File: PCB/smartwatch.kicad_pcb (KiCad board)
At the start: 2 copper layers, 34.2 x 34.2 mm, 6 parts, among them J1 Conn_01x04_Pin, U1 STM32L432KBUx, U2 LSM6DS3, U3 W25Q128JVPIQ, U4 TP4056

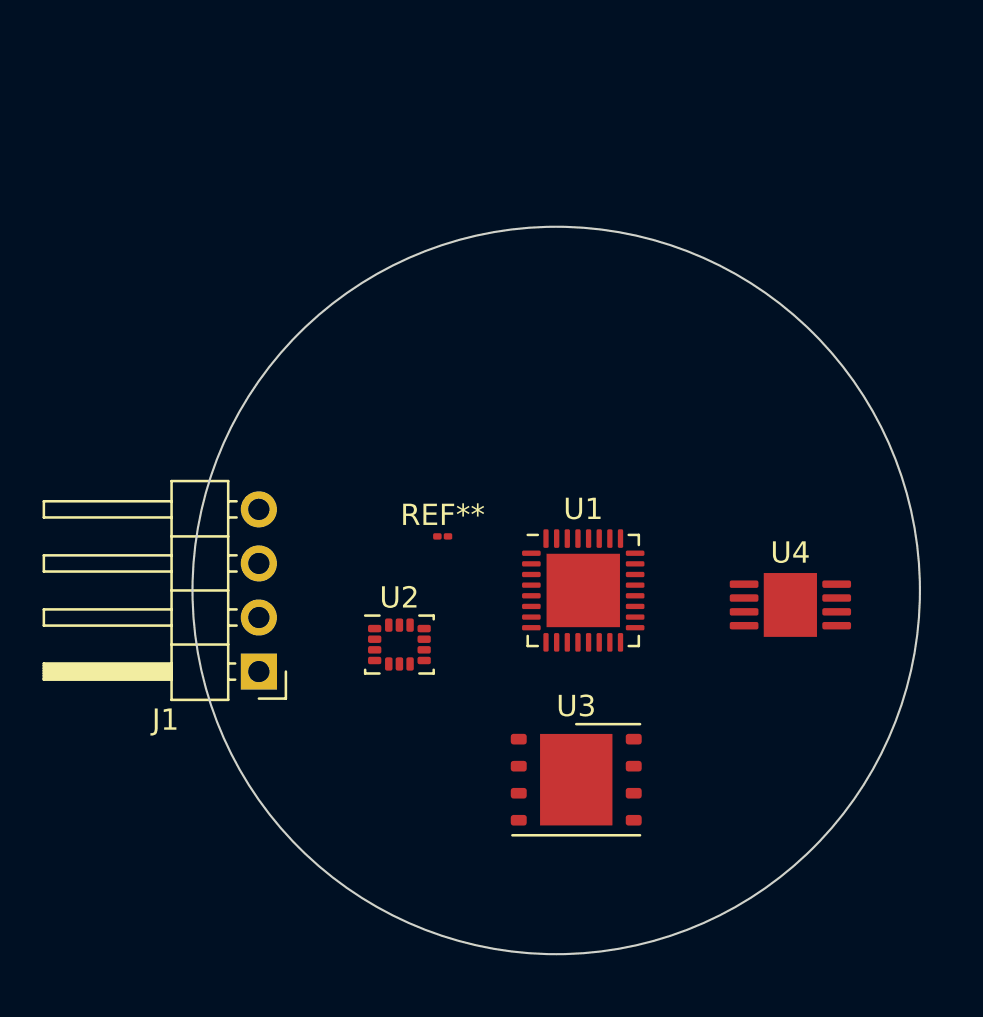
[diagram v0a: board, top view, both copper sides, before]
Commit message: new staffz
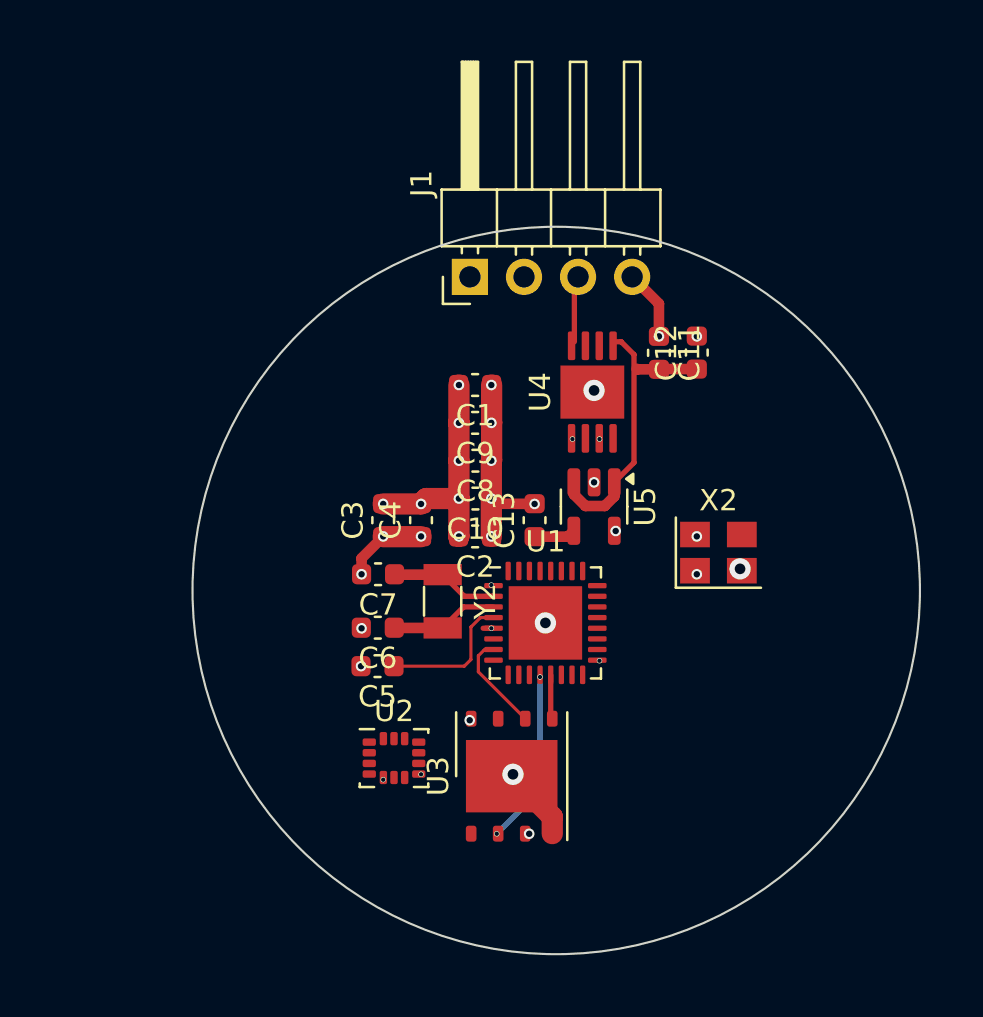
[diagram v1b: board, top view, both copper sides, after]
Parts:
- removed REF**: C_01005_0402Metric, Capacitor_SMD:C_01005_0402Metric
- added C1: 4.7uf, Capacitor_SMD:C_0603_1608Metric, F.Cu at (153.7, 84.3)
- added C10: 100nf, Capacitor_SMD:C_0603_1608Metric, F.Cu at (153.7, 89.7)
- added C11: 4.7uf, Capacitor_SMD:C_0603_1608Metric, F.Cu at (162.3, 82.8)
- added C12: 4.7uf, Capacitor_SMD:C_0603_1608Metric, F.Cu at (164.1, 82.8)
- added C13: 4.7uf, Capacitor_SMD:C_0603_1608Metric, F.Cu at (156.5, 90.7)
- added C2: 100nf, Capacitor_SMD:C_0603_1608Metric, F.Cu at (153.7, 91.4)
- added C3: 100nf, Capacitor_SMD:C_0603_1608Metric, F.Cu at (149.4, 90.7)
- added C4: 100nf, Capacitor_SMD:C_0603_1608Metric, F.Cu at (151.1, 90.7)
- added C5: 100nf, Capacitor_SMD:C_0603_1608Metric, F.Cu at (149.1, 97.5)
- added C6: 9pf, Capacitor_SMD:C_0603_1608Metric, F.Cu at (149.1, 95.7)
- added C7: 9pf, Capacitor_SMD:C_0603_1608Metric, F.Cu at (149.1, 93.2)
- added C8: 100nf, Capacitor_SMD:C_0603_1608Metric, F.Cu at (153.7, 87.9)
- added C9: 100nf, Capacitor_SMD:C_0603_1608Metric, F.Cu at (153.7, 86.1)
- added U5: LT1761-3.3, Package_TO_SOT_SMD:TSOT-23-5, F.Cu at (159.3, 90.0)
- added X2: 20Mhz, Crystal:Crystal_SMD_3225-4Pin_3.2x2.5mm, F.Cu at (165.1, 92.2)
- added Y2: LSE 32khz, Crystal:Crystal_SMD_3215-2Pin_3.2x1.5mm, F.Cu at (152.1, 94.5)
- J1: value Conn_01x04_Pin -> Serial wire/Charging
- moved J1 21.0 mm to (153.4, 79.2), turned to 90 degrees
- moved U4 13.7 mm to (159.2, 84.7), turned to 90 degrees
- moved U2 5.34 mm to (149.9, 101.9)
- moved U3 3.04 mm to (155.4, 102.7), turned to 90 degrees
- moved U1 2.34 mm to (157.0, 95.5)
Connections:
- J1 pad 3: unconnected-(J1-Pin_3-Pad3) -> VIN
- J1 pad 4: unconnected-(J1-Pin_4-Pad4) -> GND
- U1 pad 1: unconnected-(U1-VDD-Pad1) -> VDD
- U1 pad 12: unconnected-(U1-PA6-Pad12) -> SPI1_MISO
- U1 pad 13: unconnected-(U1-PA7-Pad13) -> SPI1_MOSI
- U1 pad 16: Net-(U1-VSS-Pad16) -> GND
- U1 pad 17: unconnected-(U1-VDD-Pad17) -> VDD
- U1 pad 2: unconnected-(U1-PC14-Pad2) -> OSC32_IN
- U1 pad 3: unconnected-(U1-PC15-Pad3) -> OSC32_OUT
- U1 pad 32: Net-(U1-VSS-Pad16) -> GND
- U1 pad 33: Net-(U1-VSS-Pad16) -> GND
- U1 pad 4: unconnected-(U1-NRST-Pad4) -> Net-(U1-NRST)
- U1 pad 5: unconnected-(U1-VDDA-Pad5) -> VDD
- U1 pad 6: unconnected-(U1-PA0-Pad6) -> CLKIN
- U1 pad 7: unconnected-(U1-PA1-Pad7) -> SPI1_SCK
- U2 pad 1: unconnected-(U2-SDO/SA0-Pad1) -> SPI1_MISO
- U2 pad 12: unconnected-(U2-CS-Pad12) -> GYRO_CS
- U2 pad 13: unconnected-(U2-SCL-Pad13) -> SPI1_SCK
- U2 pad 14: unconnected-(U2-SDA-Pad14) -> SPI1_MISO
- U2 pad 2: unconnected-(U2-SDX-Pad2) -> GND
- U2 pad 3: unconnected-(U2-SCX-Pad3) -> GND
- U2 pad 4: unconnected-(U2-INT1-Pad4) -> GYRO_INT1
- U2 pad 5: unconnected-(U2-VDDIO-Pad5) -> VDD
- U2 pad 6: Net-(U2-GND-Pad6) -> GND
- U2 pad 7: Net-(U2-GND-Pad6) -> GND
- U2 pad 8: unconnected-(U2-VDD-Pad8) -> VDD
- U2 pad 9: unconnected-(U2-INT2-Pad9) -> GYRO_INT2
- U3 pad 1: unconnected-(U3-/CS-Pad1) -> FLASH_CS
- U3 pad 2: unconnected-(U3-DO_(IO1)-Pad2) -> SPI1_MISO
- U3 pad 3: unconnected-(U3-/WP_(IO2)-Pad3) -> VDD
- U3 pad 4: (no net) -> GND
- U3 pad 5: unconnected-(U3-DI_(IO0)-Pad5) -> SPI1_MOSI
- U3 pad 6: unconnected-(U3-CLK-Pad6) -> SPI1_SCK
- U3 pad 7: unconnected-(U3-/HOLD_or_/RESET_(IO3)-Pad7) -> HR_FLASH
- U3 pad 8: unconnected-(U3-VCC-Pad8) -> VDD
- U3 pad 9: unconnected-(U3-Pad9) -> GND
- U4 pad 1: unconnected-(U4-TEMP-Pad1) -> GND
- U4 pad 2: unconnected-(U4-PROG-Pad2) -> Net-(U4-PROG)
- U4 pad 3: unconnected-(U4-GND-Pad3) -> GND
- U4 pad 4: unconnected-(U4-VCC-Pad4) -> VIN
- U4 pad 5: unconnected-(U4-BAT-Pad5) -> BAT
- U4 pad 7: unconnected-(U4-~{CHRG}-Pad7) -> CHARGE
- U4 pad 8: unconnected-(U4-CE-Pad8) -> VIN
- U4 pad 9: unconnected-(U4-PP-Pad9) -> GND
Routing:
- net GND: track 0.00 -> 89.1 mm, vias 0 -> 20
- net VDD: track 0.00 -> 70.5 mm, vias 0 -> 17
- net BAT: track 0.00 -> 13.9 mm
- net SPI1_MISO: track 0.00 -> 8.21 mm, vias 0 -> 2
- net Net-(U1-NRST): track 0.00 -> 6.51 mm
- net OSC32_IN: track 0.00 -> 5.08 mm
- net OSC32_OUT: track 0.00 -> 5.07 mm
- net SPI1_SCK: track 0.00 -> 4.70 mm
- net VIN: track 0.00 -> 3.12 mm
- net SPI1_MOSI: track 0.00 -> 2.09 mm
- net Net-(U5-BYP): track 0.00 -> 1.96 mm
- added copper zone on In1.Cu, net GND
- added copper zone on In2.Cu, net VDD
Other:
- copper layers 2 -> 4

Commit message: files?
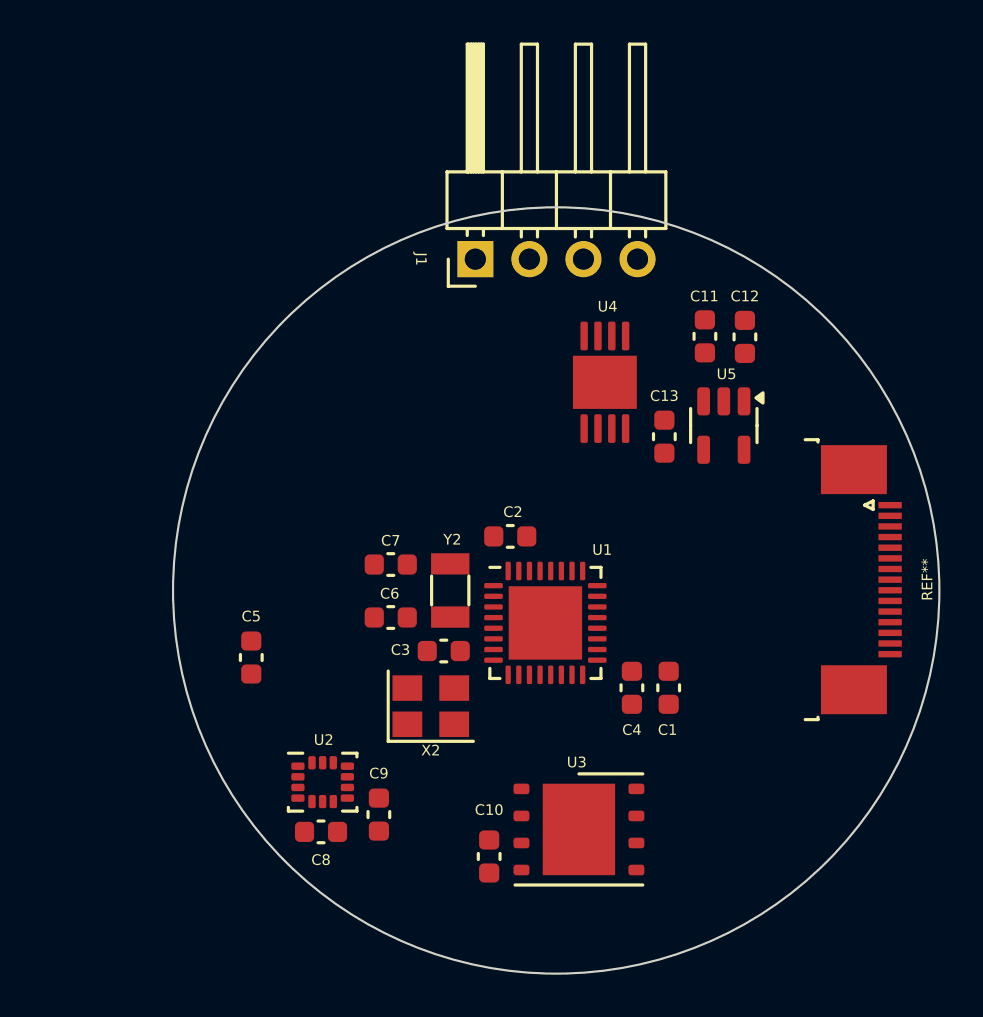
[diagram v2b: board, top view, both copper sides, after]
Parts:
- added REF**: PCB Edge, Connector_FFC-FPC:TE_1-1734839-5_1x15-1MP_P0.5mm_Horizontal, F.Cu at (171.8, 93.5)
- moved C9 18.9 mm to (149.1, 104.5), turned to 90 degrees
- moved C8 18.9 mm to (146.4, 105.3)
- moved C1 16.9 mm to (162.8, 98.6), turned to 90 degrees
- moved C10 16.8 mm to (154.3, 106.5), turned to 90 degrees
- moved X2 15.3 mm to (151.6, 99.4)
- moved C4 12.7 mm to (161.0, 98.6)
- moved C13 7.25 mm to (162.6, 86.8)
- moved U5 7.19 mm to (165.4, 86.2)
- moved C3 6.77 mm to (152.2, 96.8), turned to 0 degrees
- moved C5 5.94 mm to (143.2, 97.1), turned to -90 degrees
- moved U3 4.03 mm to (158.5, 105.2), turned to 0 degrees
- moved U2 3.54 mm to (146.5, 103.0)
- moved C12 2.38 mm to (166.3, 82.1), turned to -90 degrees
- moved C11 2.29 mm to (164.5, 82.0), turned to 90 degrees
- moved C2 1.65 mm to (155.3, 91.4)
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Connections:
- J1 pad 1: unconnected-(J1-Pin_1-Pad1) -> SWCLK
- J1 pad 2: unconnected-(J1-Pin_2-Pad2) -> SWDIO
- U1 pad 11: unconnected-(U1-PA5-Pad11) -> FLASH_SCK
- U1 pad 12: SPI1_MISO -> FLASH_MISO
- U1 pad 13: SPI1_MOSI -> FLASH_MOSI
- U1 pad 18: unconnected-(U1-PA8-Pad18) -> FLASH_CS
- U1 pad 24: unconnected-(U1-PA14-Pad24) -> SWCLK
- U1 pad 25: unconnected-(U1-PA15-Pad25) -> SWDIO
- U1 pad 26: unconnected-(U1-PB3-Pad26) -> GYRO_SCK
- U1 pad 27: unconnected-(U1-PB4-Pad27) -> GYRO_MISO
- U1 pad 28: unconnected-(U1-PB5-Pad28) -> GYRO_MOSI
- U1 pad 29: unconnected-(U1-PB6-Pad29) -> GYRO_CS
- U1 pad 7: SPI1_SCK -> BAT
- U2 pad 1: SPI1_MISO -> GYRO_MISO
- U2 pad 13: SPI1_SCK -> GYRO_SCK
- U2 pad 14: SPI1_MISO -> GYRO_MOSI
- U3 pad 2: SPI1_MISO -> FLASH_MISO
- U3 pad 6: SPI1_SCK -> FLASH_SCK
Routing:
- net GND: track 89.1 -> 0.00 mm, vias 20 -> 0
- net VDD: track 70.5 -> 0.00 mm, vias 17 -> 0
- net BAT: track 13.9 -> 0.00 mm
- net SPI1_MISO: track 8.21 -> 0.00 mm, vias 2 -> 0
- net Net-(U1-NRST): track 6.51 -> 0.00 mm
- net OSC32_IN: track 5.08 -> 0.00 mm
- net OSC32_OUT: track 5.07 -> 0.00 mm
- net SPI1_SCK: track 4.70 -> 0.00 mm
- net VIN: track 3.12 -> 0.00 mm
- net SPI1_MOSI: track 2.09 -> 0.00 mm
- net Net-(U5-BYP): track 1.96 -> 0.00 mm
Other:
- board size 34.2 x 34.2 mm -> 36 x 36 mm
